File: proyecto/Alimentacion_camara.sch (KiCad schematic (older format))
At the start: 9 parts

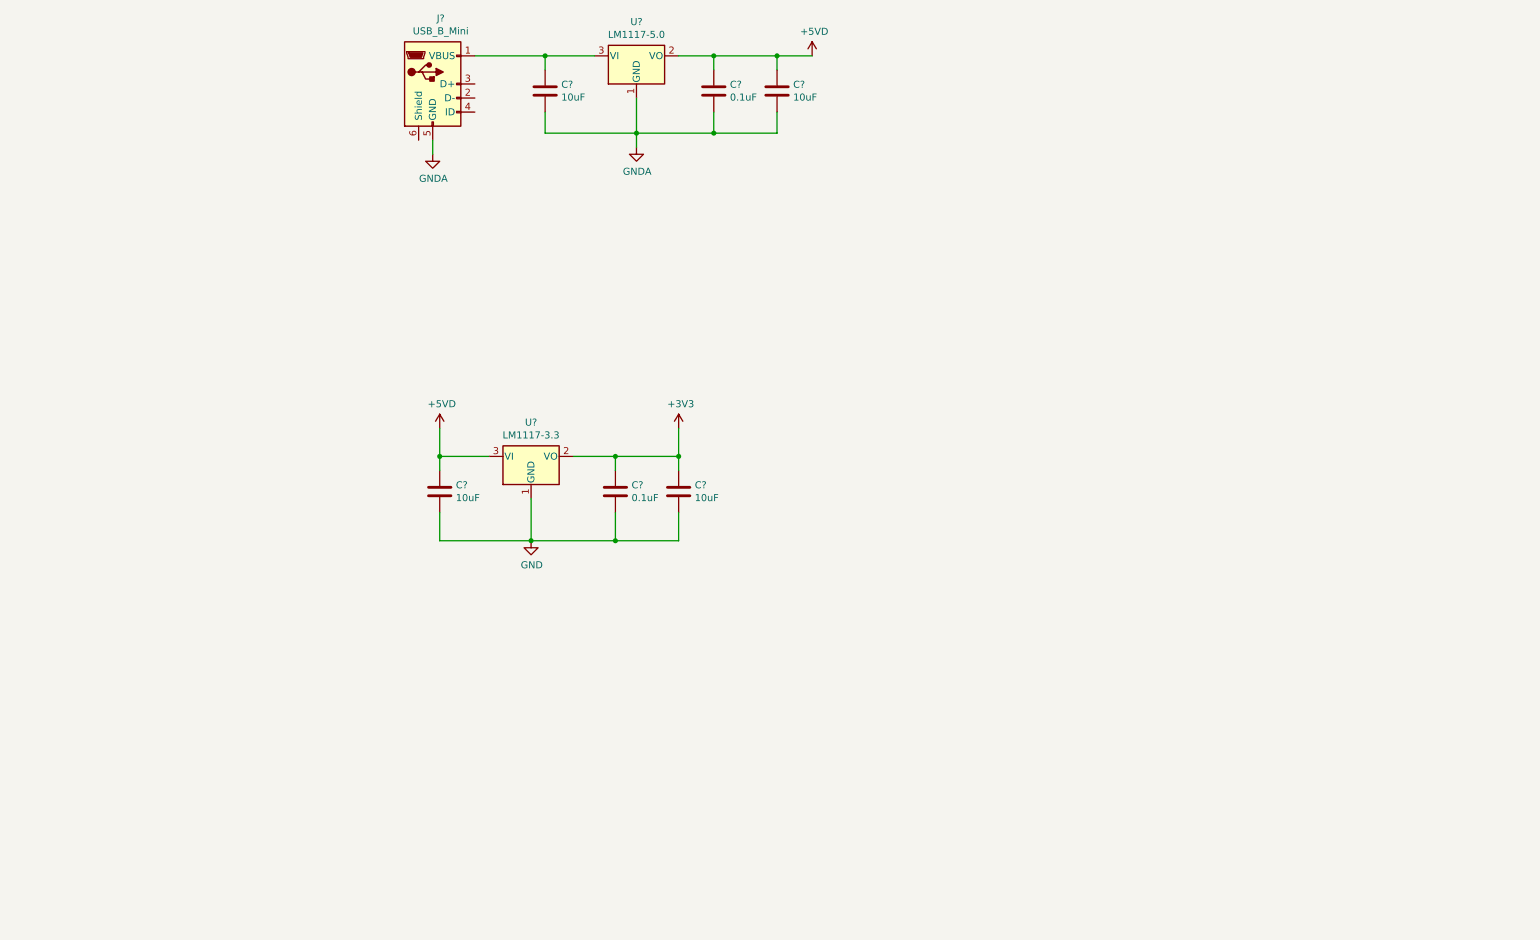
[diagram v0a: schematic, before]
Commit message: Add files via upload
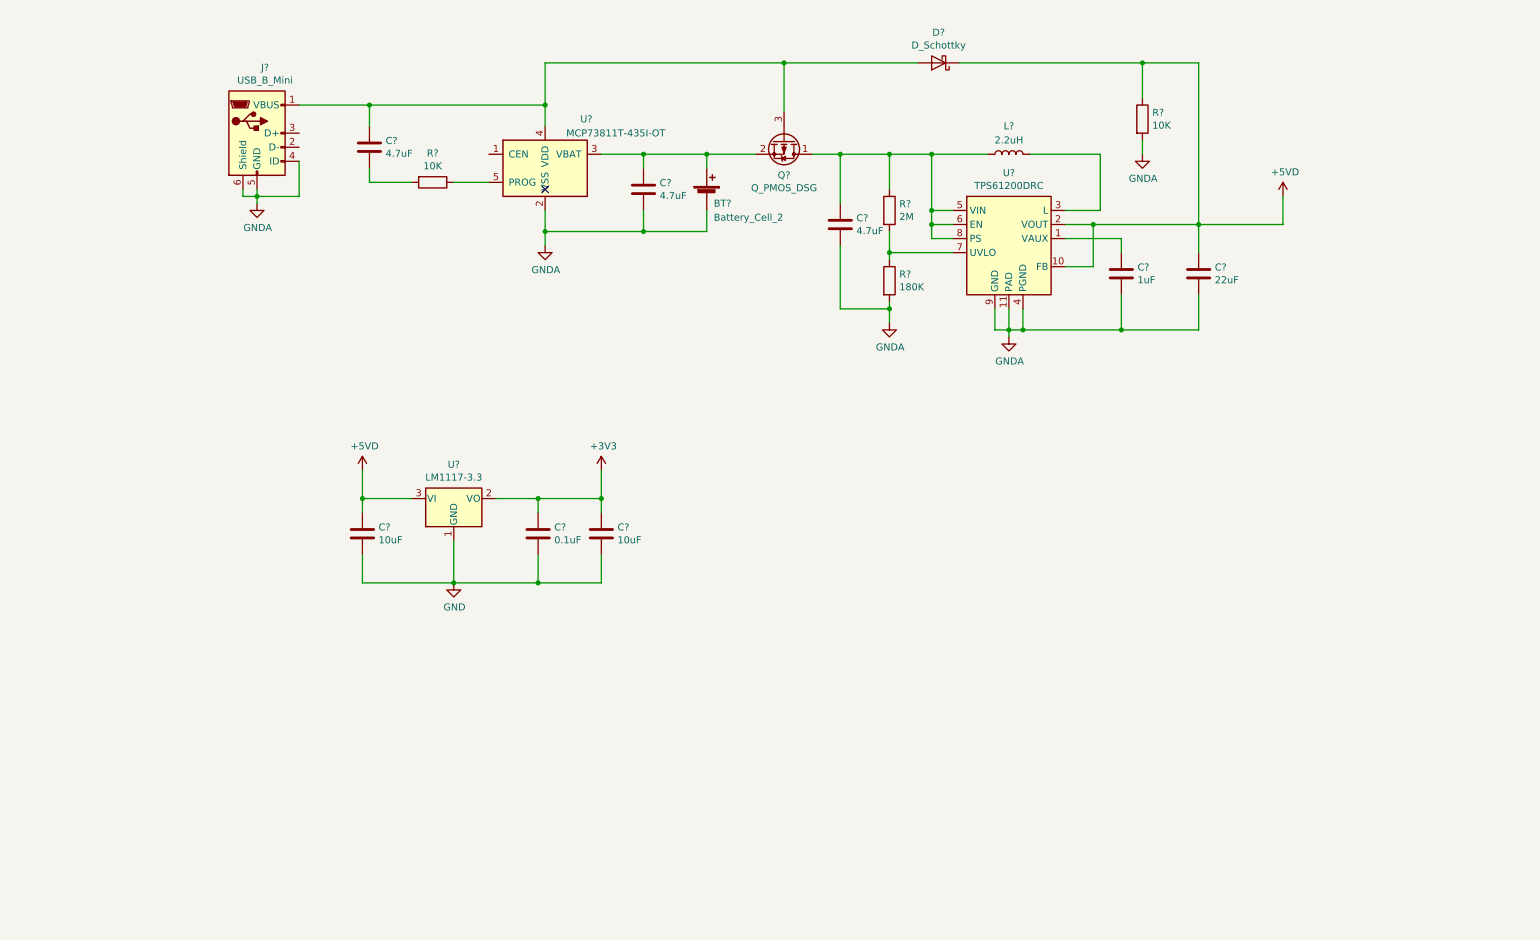
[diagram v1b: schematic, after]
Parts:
- removed C?: 0.1uF, symbol Device:C
- removed C? (x2): 10uF, symbol Device:C
- removed U?: LM1117-5.0, symbol Regulator_Linear:LM1117-5.0
- added BT?: Battery_Cell_2, symbol Device:Battery_Cell
- added C? (x3): 4.7uF, symbol Device:C
- added C?: 1uF, symbol Device:C
- added C?: 22uF, symbol Device:C
- added D?: D_Schottky, symbol Device:D_Schottky
- added L?: 2.2uH, symbol Device:L
- added Q?: Q_PMOS_DSG, symbol Device:Q_PMOS_DSG
- added R? (x2): 10K, symbol Device:R
- added R?: 2M, symbol Device:R
- added R?: 180K, symbol Device:R
- added U?: MCP73811T-435I-OT, Package_TO_SOT_SMD:SOT-23-5, symbol Battery_Management:MCP73811T-435I-OT
- added U?: TPS61200DRC, Package_SON:Texas_S-PVSON-N10_ThermalVias, symbol Regulator_Switching:TPS61200DRC
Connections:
- net +5VD: now also C?.1, D?.1 (K), R?.1, U?.10 (FB), U?.2 (VOUT)
- net GNDA: now also J?.4 (ID), J?.6 (Shield), BT?.2 (-), C?.2, C?.2, C?.2, C?.2, R?.2, R?.2, U?.11 (PAD), U?.2 (VSS), U?.4 (PGND), U?.9 (GND)
- net at J?.1 (VBUS): now also C?.1, D?.2 (A), Q?.3 (G), U?.4 (VDD)
- new net: C?.2, R?.2
- new net: R?.1, U?.5 (PROG)
- new net: BT?.1 (+), C?.1, Q?.2 (S), U?.3 (VBAT)
- new net: C?.1, L?.1, Q?.1 (D), R?.1, U?.5 (VIN), U?.6 (EN), U?.8 (PS)
- new net: C?.1, U?.1 (VAUX)
- new net: L?.2, U?.3 (L)
- new net: R?.1, R?.2, U?.7 (UVLO)
- no-connect marks 0 -> 1
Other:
- moved on the sheet: C?, J?, U?

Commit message: Add files via upload
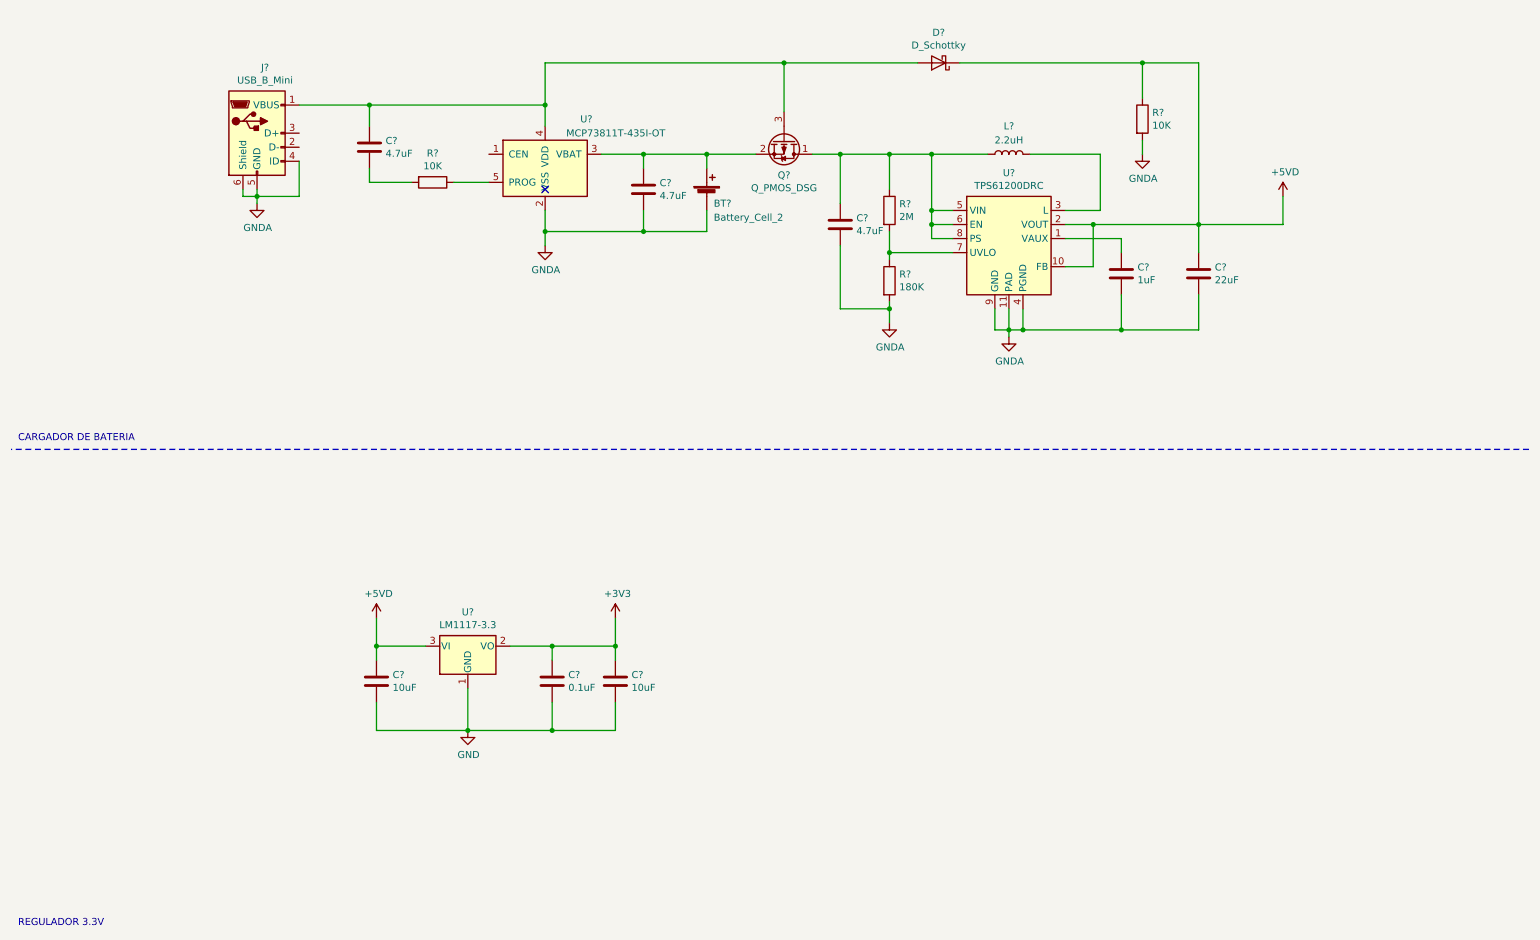
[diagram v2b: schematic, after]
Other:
- note added: "CARGADOR DE BATERIA"
- note added: "REGULADOR 3.3V"
- moved on the sheet: C?, U?
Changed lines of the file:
@@
 Comment4 ""
 $EndDescr
-$Comp
-L Regulator_Linear:LM1117-3.3 U?
-U 1 1 5E9D90F6
-P 3600 4700
-AR Path="/5E9D90F6" Ref="U?"  Part="1"
-AR Path="/5E9BC166/5E9D90F6" Ref="U?"  Part="1"
-AR Path="/5EA3D59C/5E9D90F6" Ref="U?"  Part="1"
-F 0 "U?" H 3600 4942 50  0000 C CNN
-F 1 "LM1117-3.3" H 3600 4851 50  0000 C CNN
-F 2 "" H 3600 4700 50  0001 C CNN
-F 3 "http://www.ti.com/lit/ds/symlink/lm1117.pdf" H 3600 4700 50  0001 C CNN
-	1    3600 4700
-	1    0    0    -1
-$EndComp
-$Comp
-L Device:C C?
-U 1 1 5E9D90FC
-P 2950 4950
-AR Path="/5E9D90FC" Ref="C?"  Part="1"
-AR Path="/5E9BC166/5E9D90FC" Ref="C?"  Part="1"
-AR Path="/5EA3D59C/5E9D90FC" Ref="C?"  Part="1"
-F 0 "C?" H 3065 4996 50  0000 L CNN
-F 1 "10uF" H 3065 4905 50  0000 L CNN
-F 2 "" H 2988 4800 50  0001 C CNN
-F 3 "~" H 2950 4950 50  0001 C CNN
-	1    2950 4950
-	1    0    0    -1
-$EndComp
-$Comp
-L Device:C C?
-U 1 1 5E9D9102
-P 4200 4950
-AR Path="/5E9D9102" Ref="C?"  Part="1"
-AR Path="/5E9BC166/5E9D9102" Ref="C?"  Part="1"
-AR Path="/5EA3D59C/5E9D9102" Ref="C?"  Part="1"
-F 0 "C?" H 4315 4996 50  0000 L CNN
-F 1 "0.1uF" H 4315 4905 50  0000 L CNN
-F 2 "" H 4238 4800 50  0001 C CNN
-F 3 "~" H 4200 4950 50  0001 C CNN
-	1    4200 4950
-	1    0    0    -1
-$EndComp
-$Comp
-L Device:C C?
-U 1 1 5E9D9108
-P 4650 4950
-AR Path="/5E9D9108" Ref="C?"  Part="1"
-AR Path="/5E9BC166/5E9D9108" Ref="C?"  Part="1"
-AR Path="/5EA3D59C/5E9D9108" Ref="C?"  Part="1"
-F 0 "C?" H 4765 4996 50  0000 L CNN
-F 1 "10uF" H 4765 4905 50  0000 L CNN
-F 2 "" H 4688 4800 50  0001 C CNN
-F 3 "~" H 4650 4950 50  0001 C CNN
-	1    4650 4950
-	1    0    0    -1
-$EndComp
-Wire Wire Line
-	3300 4700 2950 4700
-Wire Wire Line
-	2950 4800 2950 4700
-Wire Wire Line
-	4200 4800 4200 4700
-Connection ~ 4200 4700
-Wire Wire Line
-	4200 4700 3900 4700
-Wire Wire Line
-	4650 4800 4650 4700
-Wire Wire Line
-	4650 4700 4200 4700
-$Comp
-L power:GND #PWR?
-U 1 1 5E9D911B
-P 3600 5300
-AR Path="/5E9D911B" Ref="#PWR?"  Part="1"
-AR Path="/5E9BC166/5E9D911B" Ref="#PWR?"  Part="1"
-AR Path="/5EA3D59C/5E9D911B" Ref="#PWR?"  Part="1"
-F 0 "#PWR?" H 3600 5050 50  0001 C CNN
-F 1 "GND" H 3605 5127 50  0000 C CNN
-F 2 "" H 3600 5300 50  0001 C CNN
-F 3 "" H 3600 5300 50  0001 C CNN
-	1    3600 5300
-	1    0    0    -1
-$EndComp
-Wire Wire Line
-	4650 5300 4200 5300
-Connection ~ 3600 5300
-Wire Wire Line
-	3600 5000 3600 5300
-Wire Wire Line
-	4200 5100 4200 5300
-Connection ~ 4200 5300
-Wire Wire Line
-	4200 5300 3600 5300
-Wire Wire Line
-	2950 5100 2950 5300
-Wire Wire Line
-	2950 5300 3600 5300
-Wire Wire Line
-	4650 5100 4650 5300
-Wire Wire Line
-	4650 4500 4650 4700
-Connection ~ 4650 4700
-Wire Wire Line
-	2950 4700 2950 4500
-Connection ~ 2950 4700
-$Comp
-L power:+5VD #PWR?
-U 1 1 5EA5E622
-P 2950 4500
-F 0 "#PWR?" H 2950 4350 50  0001 C CNN
-F 1 "+5VD" H 2965 4673 50  0000 C CNN
-F 2 "" H 2950 4500 50  0001 C CNN
-F 3 "" H 2950 4500 50  0001 C CNN
-	1    2950 4500
-	1    0    0    -1
-$EndComp
+Wire Wire Line
+	4750 6150 4750 6350
 $Comp
 L power:+3V3 #PWR?
 U 1 1 5EA5F12F
-P 4650 4500
-F 0 "#PWR?" H 4650 4350 50  0001 C CNN
-F 1 "+3V3" H 4665 4673 50  0000 C CNN
-F 2 "" H 4650 4500 50  0001 C CNN
-F 3 "" H 4650 4500 50  0001 C CNN
-	1    4650 4500
+P 4750 5550
+F 0 "#PWR?" H 4750 5400 50  0001 C CNN
+F 1 "+3V3" H 4765 5723 50  0000 C CNN
+F 2 "" H 4750 5550 50  0001 C CNN
+F 3 "" H 4750 5550 50  0001 C CNN
+	1    4750 5550
 	1    0    0    -1
 $EndComp
@@
 	1    0    0    -1
 $EndComp
+Connection ~ 4750 5750
+Wire Wire Line
+	4750 5550 4750 5750
+Wire Wire Line
+	4750 5850 4750 5750
+$Comp
+L power:+5VD #PWR?
+U 1 1 5EA5E622
+P 3050 5550
+F 0 "#PWR?" H 3050 5400 50  0001 C CNN
+F 1 "+5VD" H 3065 5723 50  0000 C CNN
+F 2 "" H 3050 5550 50  0001 C CNN
+F 3 "" H 3050 5550 50  0001 C CNN
+	1    3050 5550
+	1    0    0    -1
+$EndComp
+Connection ~ 3050 5750
+Wire Wire Line
+	3050 5750 3050 5550
+Wire Wire Line
+	3050 6350 3700 6350
+Wire Wire Line
+	3050 6150 3050 6350
+Wire Wire Line
+	4300 6350 3700 6350
+Connection ~ 4300 6350
+Wire Wire Line
+	4300 6150 4300 6350
+Wire Wire Line
+	3700 6050 3700 6350
+Connection ~ 3700 6350
+Wire Wire Line
+	4750 6350 4300 6350
+$Comp
+L power:GND #PWR?
+U 1 1 5E9D911B
+P 3700 6350
+AR Path="/5E9D911B" Ref="#PWR?"  Part="1"
+AR Path="/5E9BC166/5E9D911B" Ref="#PWR?"  Part="1"
+AR Path="/5EA3D59C/5E9D911B" Ref="#PWR?"  Part="1"
+F 0 "#PWR?" H 3700 6100 50  0001 C CNN
+F 1 "GND" H 3705 6177 50  0000 C CNN
+F 2 "" H 3700 6350 50  0001 C CNN
+F 3 "" H 3700 6350 50  0001 C CNN
+	1    3700 6350
+	1    0    0    -1
+$EndComp
+Wire Wire Line
+	4750 5750 4300 5750
+Wire Wire Line
+	4300 5750 4000 5750
+Connection ~ 4300 5750
+Wire Wire Line
+	4300 5850 4300 5750
+Wire Wire Line
+	3050 5850 3050 5750
+Wire Wire Line
+	3400 5750 3050 5750
+$Comp
+L Device:C C?
+U 1 1 5E9D9108
+P 4750 6000
+AR Path="/5E9D9108" Ref="C?"  Part="1"
+AR Path="/5E9BC166/5E9D9108" Ref="C?"  Part="1"
+AR Path="/5EA3D59C/5E9D9108" Ref="C?"  Part="1"
+F 0 "C?" H 4865 6046 50  0000 L CNN
+F 1 "10uF" H 4865 5955 50  0000 L CNN
+F 2 "" H 4788 5850 50  0001 C CNN
+F 3 "~" H 4750 6000 50  0001 C CNN
+	1    4750 6000
+	1    0    0    -1
+$EndComp
+$Comp
+L Device:C C?
+U 1 1 5E9D9102
+P 4300 6000
+AR Path="/5E9D9102" Ref="C?"  Part="1"
+AR Path="/5E9BC166/5E9D9102" Ref="C?"  Part="1"
+AR Path="/5EA3D59C/5E9D9102" Ref="C?"  Part="1"
+F 0 "C?" H 4415 6046 50  0000 L CNN
+F 1 "0.1uF" H 4415 5955 50  0000 L CNN
+F 2 "" H 4338 5850 50  0001 C CNN
+F 3 "~" H 4300 6000 50  0001 C CNN
+	1    4300 6000
+	1    0    0    -1
+$EndComp
+$Comp
+L Device:C C?
+U 1 1 5E9D90FC
+P 3050 6000
+AR Path="/5E9D90FC" Ref="C?"  Part="1"
+AR Path="/5E9BC166/5E9D90FC" Ref="C?"  Part="1"
+AR Path="/5EA3D59C/5E9D90FC" Ref="C?"  Part="1"
+F 0 "C?" H 3165 6046 50  0000 L CNN
+F 1 "10uF" H 3165 5955 50  0000 L CNN
+F 2 "" H 3088 5850 50  0001 C CNN
+F 3 "~" H 3050 6000 50  0001 C CNN
+	1    3050 6000
+	1    0    0    -1
+$EndComp
+$Comp
+L Regulator_Linear:LM1117-3.3 U?
+U 1 1 5E9D90F6
+P 3700 5750
+AR Path="/5E9D90F6" Ref="U?"  Part="1"
+AR Path="/5E9BC166/5E9D90F6" Ref="U?"  Part="1"
+AR Path="/5EA3D59C/5E9D90F6" Ref="U?"  Part="1"
+F 0 "U?" H 3700 5992 50  0000 C CNN
+F 1 "LM1117-3.3" H 3700 5901 50  0000 C CNN
+F 2 "" H 3700 5750 50  0001 C CNN
+F 3 "http://www.ti.com/lit/ds/symlink/lm1117.pdf" H 3700 5750 50  0001 C CNN
+	1    3700 5750
+	1    0    0    -1
+$EndComp
+Wire Notes Line
+	11250 4350 450  4350
+Text Notes 500  4300 0    50   ~ 0
+CARGADOR DE BATERIA
+Text Notes 500  7750 0    50   ~ 0
+REGULADOR 3.3V
 $EndSCHEMATC
